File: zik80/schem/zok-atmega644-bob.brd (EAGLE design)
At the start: 99.1 x 99.1 mm, 45 parts, among them IC1 TPS7133QP, U2 FT232RLSSOP

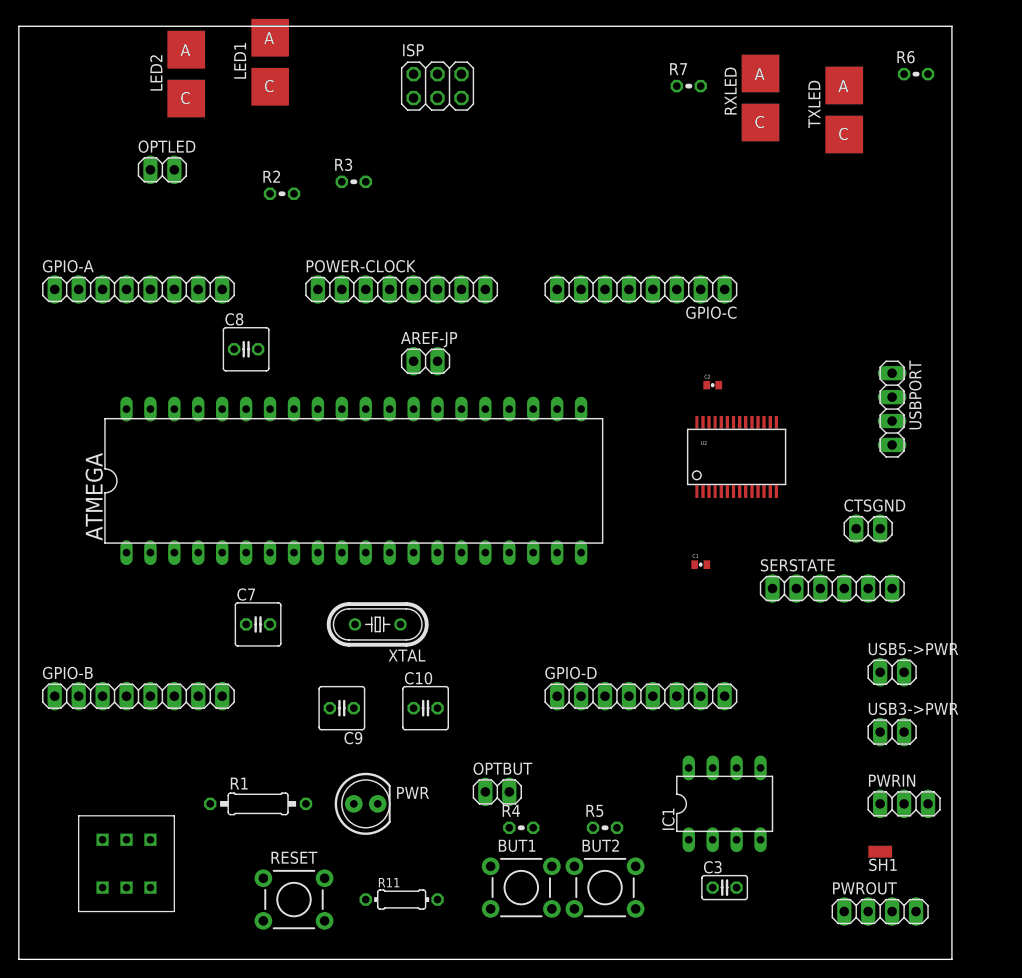
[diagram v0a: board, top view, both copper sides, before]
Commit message: Finished up zok atmega bob rev1, and zikzak sbc rev3
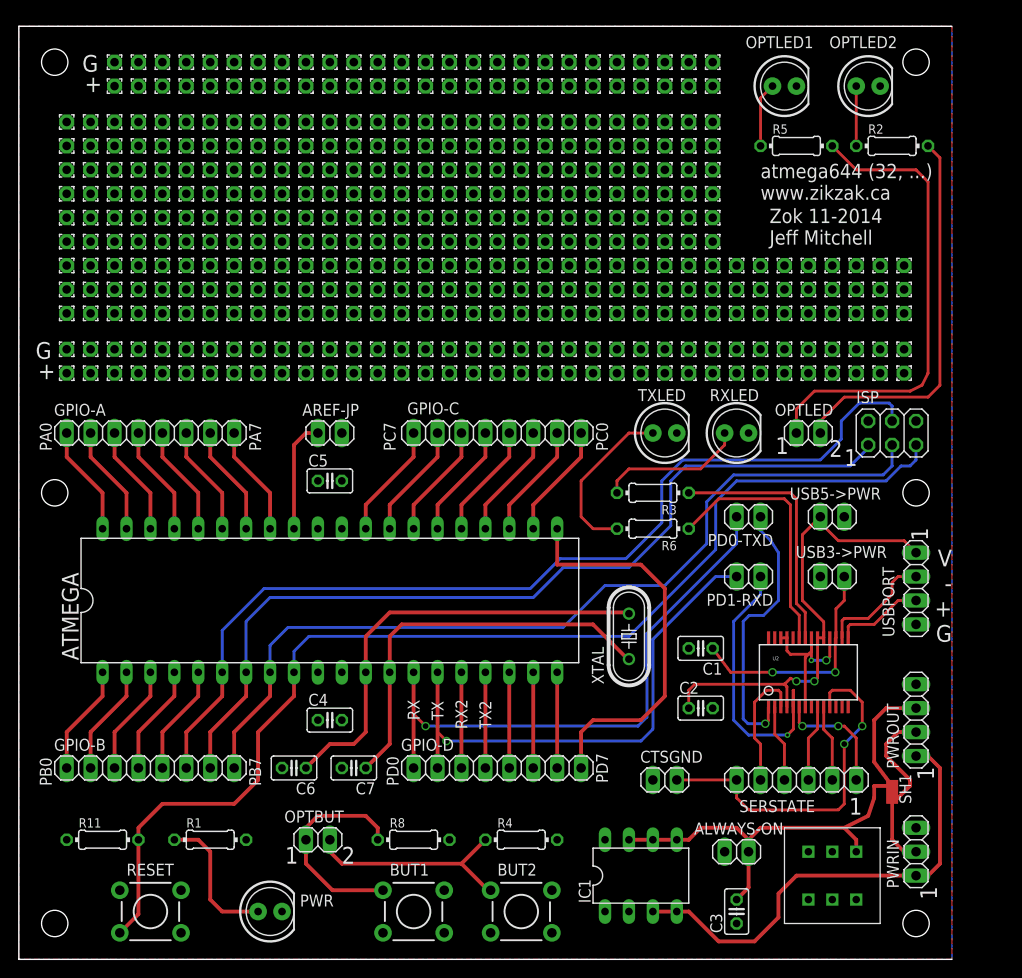
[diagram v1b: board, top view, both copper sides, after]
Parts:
- removed C10, C9: 22pf, rcl:C025-050X050
- removed C8: (no value), rcl:C025-050X050
- removed LED1, LED2: (no value), led:OSRAM-MINI-TOP-LED
- removed POWER-CLOCK: (no value), pinhead:1X08
- removed R7: (no value), rcl:0204V
- added ALWAYS-ON, PD0-TXD, PD1-RXD: (no value), pinhead:1X02
- added C4, C5: .1uF, rcl:C025-025X050
- added C6: 22pF, rcl:C025-025X050
- added OPTLED1, OPTLED2: (no value), SparkFun-LED:LED5MM
- added P1, P10, P100, P101, P102, P103, P104, P105, P106, P107, P108, P109, P11, P110, P111, P112, P113, P114, P115, P116, P117, P118, P119, P12, P120, P121, P122, P123, P124, P125, P126, P127, P128, P129, P13, P130, P139, P14, P140, P141, P142, P143, P144, P145, P146, P147, P148, P149, P15, P150, P151, P152, P153, P154, P155, P156, P157, P158, P159, P16, P160, P161, P162, P163, P164, P165, P166, P167, P168, P169, P17, P170, P171, P172, P173, P174, P175, P176, P177, P178, P179, P18, P180, P183, P184, P185, P186, P187, P188, P189, P19, P190, P191, P192, P193, P194, P195, P196, P197, P198, P199, P2, P20, P200, P201, P202, P203, P204, P205, P206, P207, P208, P21, P211, P212, P213, P214, P215, P216, P217, P218, P219, P22, P220, P221, P222, P223, P224, P225, P226, P227, P228, P229, P23, P230, P231, P232, P233, P234, P235, P236, P237, P238, P239, P24, P240, P241, P242, P243, P244, P245, P246, P247, P248, P249, P25, P250, P251, P252, P253, P254, P255, P256, P257, P258, P259, P26, P260, P261, P262, P263, P264, P265, P266, P267, P268, P269, P27, P270, P271, P272, P273, P274, P275, P276, P277, P278, P279, P28, P280, P281, P282, P283, P284, P285, P286, P287, P288, P289, P29, P290, P291, P292, P293, P294, P295, P296, P297, P298, P299, P3, P30, P300, P301, P302, P303, P304, P305, P306, P307, P308, P309, P31, P310, P311, P312, P313, P314, P315, P316, P317, P318, P319, P32, P320, P321, P322, P323, P324, P325, P326, P327, P328, P329, P33, P330, P331, P332, P333, P334, P335, P336, P337, P338, P339, P34, P340, P341, P342, P343, P344, P345, P346, P347, P348, P349, P35, P350, P351, P352, P353, P354, P355, P356, P357, P358, P359, P36, P360, P361, P362, P363, P364, P365, P366, P367, P368, P369, P37, P370, P371, P372, P373, P374, P375, P376, P377, P378, P379, P38, P380, P381, P382, P383, P384, P385, P386, P387, P388, P389, P39, P390, P391, P392, P393, P394, P395, P396, P397, P398, P399, P4, P40, P400, P401, P402, P403, P404, P405, P406, P407, P408, P409, P41, P410, P411, P412, P42, P43, P44, P45, P46, P47, P48, P49, P5, P50, P51, P52, P53, P54, P55, P56, P57, P58, P59, P6, P60, P61, P62, P63, P64, P65, P66, P67, P68, P69, P7, P70, P71, P72, P73, P74, P75, P76, P77, P78, P79, P8, P80, P81, P82, P83, P84, P85, P86, P87, P88, P89, P9, P90, P91, P92, P93, P94, P95, P96, P97, P98, P99: (no value), wirepad:1,6/0,9
- added R8: 10K, rcl:0204/7
- C1, C2: value 0.1uF -> .1uF; device SparkFun:0402-CAP -> rcl:C025-025X050
- C7: value (none) -> 22pF; device rcl:C025-050X050 -> rcl:C025-025X050
- R1: device rcl:0207/10 -> rcl:0204/7
- R2, R3, R6: value (none) -> 330 ohm; device rcl:0204V -> rcl:0204/7
- R4: device rcl:0204V -> rcl:0204/7
- R5: value 10K -> 330 ohm; device rcl:0204V -> rcl:0204/7
- RXLED, TXLED: device led:OSRAM-MINI-TOP-LED -> SparkFun-LED:LED5MM
- moved R5 75.2 mm to (82.5, 86.4)
- moved U$4 74.9 mm to (81.3, 3.81)
- moved OPTLED 74.1 mm to (83.8, 55.9)
- moved R2 65.0 mm to (92.7, 86.4)
- moved ISP 60.7 mm to (92.7, 55.9)
- moved R6 55.8 mm to (67.3, 45.7), turned to 180 degrees
- moved R3 45.8 mm to (67.3, 49.5), turned to 180 degrees
- moved TXLED 39.2 mm to (68.6, 55.9)
- moved RXLED 35.7 mm to (76.2, 55.9)
- moved C2 34.3 mm to (72.4, 26.7)
- moved CTSGND 34.3 mm to (68.6, 19.1)
- moved R11 32.4 mm to (8.89, 12.7)
- moved XTAL 26.7 mm to (64.8, 34.3), turned to 90 degrees
- moved U2 24.1 mm to (83.8, 30.5)
- moved GPIO-C 21.6 mm to (50.8, 55.9)
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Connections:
- new net N$12: PD0-TXD.1, U2.1
- new net N$13: PD1-RXD.1, U2.5
- net +5V: now also ALWAYS-ON.2
- net AREF: no longer POWER-CLOCK.8
- net AT_RESET: no longer POWER-CLOCK.1
- net GND: now also C4.2, C5.2, C6.2, OPTLED1.K, OPTLED2.K, P1.1, P10.1, P11.1, P12.1, P13.1, P14.1, P15.1, P16.1, P17.1, P18.1, P183.1, P184.1, P185.1, P186.1, P187.1, P188.1, P189.1, P19.1, P190.1, P191.1, P192.1, P193.1, P194.1, P195.1, P196.1, P197.1, P198.1, P199.1, P2.1, P20.1, P200.1, P201.1, P202.1, P203.1, P204.1, P205.1, P206.1, P207.1, P208.1, P21.1, P22.1, P23.1, P24.1, P25.1, P26.1, P27.1, P28.1, P29.1, P3.1, P30.1, P31.1, P32.1, P33.1, P34.1, P35.1, P36.1, P4.1, P5.1, P6.1, P7.1, P8.1, P9.1, RXLED.K, TXLED.K; no longer C10.2, C8.2, C9.2, LED1.C, LED2.C, POWER-CLOCK.3, POWER-CLOCK.7, RXLED.C, TXLED.C
- net N$1: now also R8.1; no longer R4.2
- net N$10: now also R3.2; no longer R7.1
- net N$11: now also R3.1; no longer R7.2
- net N$2: now also R4.1; no longer R5.2
- net N$3: now also R1.1; no longer R1.2
- net N$4: now also R6.2; no longer R6.1
- net N$5: now also R5.2; no longer R2.2
- net N$6: now also OPTLED2.A, R2.1; no longer LED2.A, R3.1
- net N$7: now also R2.2; no longer R3.2
- net N$8: now also R6.1; no longer R6.2
- net N$9: now also OPTLED1.A, R5.1; no longer LED1.A, R2.1
- net PD0: now also PD0-TXD.2; no longer U2.1
- net PD1: now also PD1-RXD.2; no longer U2.5
- net PWR: now also ALWAYS-ON.1, C4.1, C5.1, P108.1, P109.1, P110.1, P111.1, P112.1, P211.1, P212.1, P213.1, P214.1, P215.1, P216.1, P217.1, P218.1, P219.1, P220.1, P221.1, P222.1, P223.1, P224.1, P225.1, P226.1, P227.1, P228.1, P229.1, P230.1, P231.1, P232.1, P233.1, P234.1, P235.1, P236.1, P37.1, P38.1, P39.1, P40.1, P41.1, P62.1, P64.1, P71.1, P74.1, P78.1, P79.1, P80.1, P81.1, P82.1, P83.1, P84.1, P85.1, P86.1, P87.1, P88.1, P89.1, P90.1, P91.1, P92.1, P93.1, P94.1, P95.1, P96.1, P97.1, P98.1, P99.1, R1.2, R4.2, R8.2; no longer C7.1, C8.1, POWER-CLOCK.2, POWER-CLOCK.6, R1.1, R4.1, R5.1
- net XTAL1: now also C7.1; no longer C10.1, POWER-CLOCK.5
- net XTAL2: now also C6.1; no longer C9.1, POWER-CLOCK.4
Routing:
- net AT_RESET: track 0.00 -> 121.0 mm
- net AT_MOSI: track 0.00 -> 102.7 mm
- net AT_MISO: track 0.00 -> 93.9 mm
- net AT_SCK: track 0.00 -> 93.4 mm
- net PD0: track 0.00 -> 65.5 mm, vias 0 -> 1
- net PD1: track 0.00 -> 61.5 mm, vias 0 -> 1
- net +5V: track 0.00 -> 55.0 mm
- net USB5: track 0.00 -> 50.4 mm, vias 0 -> 2
- net N$5: track 0.00 -> 50.3 mm
- net VCC: track 0.00 -> 49.9 mm
- net XTAL2: track 0.00 -> 47.1 mm
- net XTAL1: track 0.00 -> 42.5 mm
- net PD7: track 0.00 -> 42.0 mm
- net N$7: track 0.00 -> 41.5 mm
- net CTS: track 0.00 -> 37.6 mm, vias 0 -> 2
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- added copper zone on layer 16, net GND
- added copper zone on layer 1, net PWR
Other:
- board text added: "+"
- board text added: "1"
- board text added: "2"
- board text added: "G"
- board text added: "PA0"
- board text added: "PA7"
- board text added: "PB0"
- board text added: "PB7"
- board text added: "PC0"
- board text added: "PC7"
- board text added: "PD0"
- board text added: "PD7"
- board text added: "RX"
- board text added: "RX2"
- board text added: "TX"
- board text added: "TX2"
- board text added: "V - + G"
- board text added: "Zok 11-2014 Jeff Mitchell"
- board text added: "atmega644 (32, ...) www.zikzak.ca"
